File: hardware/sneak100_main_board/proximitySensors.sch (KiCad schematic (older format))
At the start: 29 parts, among them Q1 Q_Photo_NPN_CE, U1 CD4051B, U2 CD4051B

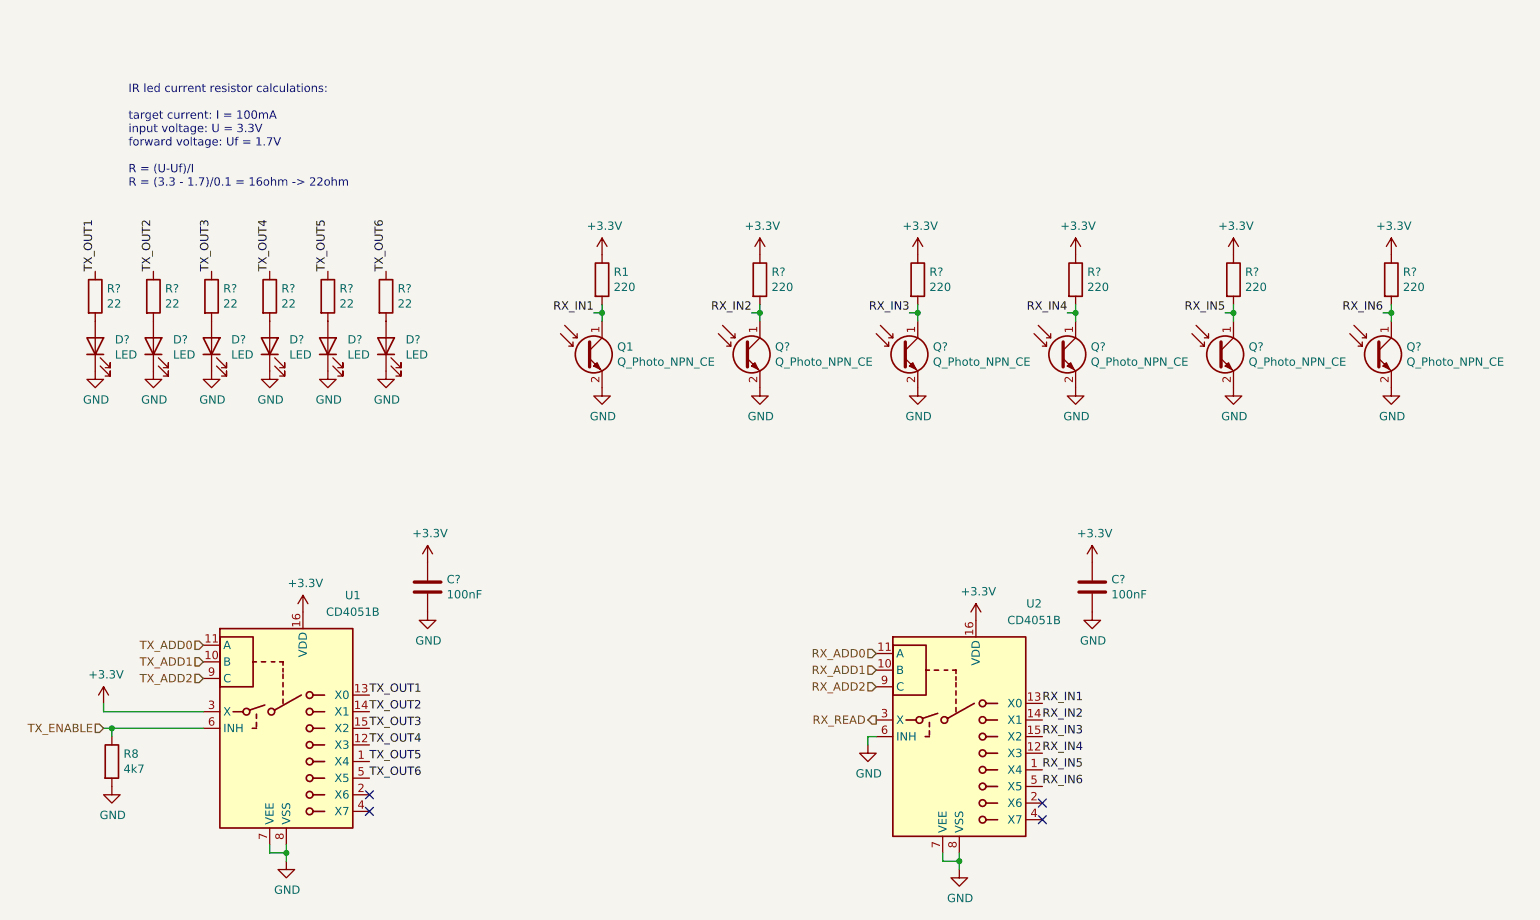
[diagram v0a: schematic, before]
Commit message: Proximity sensor first test
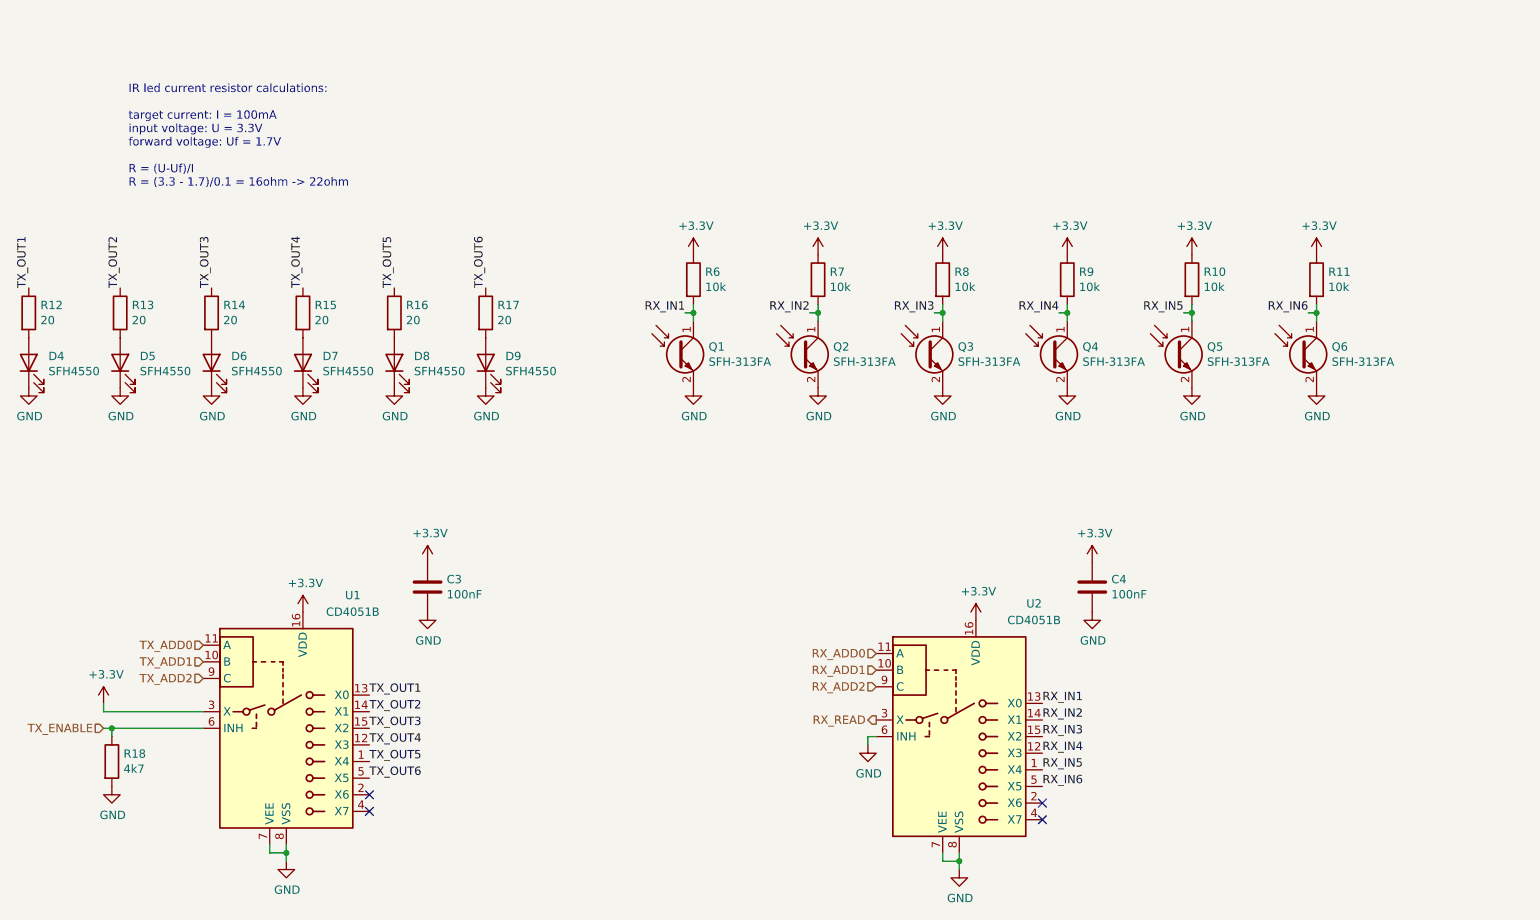
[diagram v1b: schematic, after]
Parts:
- D4, D5, D6, D7, D8, D9: renamed from D?; value LED -> SFH4550
- Q1: value Q_Photo_NPN_CE -> SFH-313FA
- Q2, Q3, Q4, Q5, Q6: renamed from Q?; value Q_Photo_NPN_CE -> SFH-313FA
- R10, R11, R7, R8, R9: renamed from R?; value 220 -> 10k
- R12, R13, R14, R15, R16, R17: renamed from R?; value 22 -> 20
- R6: renamed from R1; value 220 -> 10k
- gave numbers to parts that had none: 2
- renumbered R8 to R18
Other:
- moved on the sheet: D4, D5, D6, D7, D8, D9, Q1, Q2, Q3, Q4, Q5, Q6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

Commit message: motors circuit scheme
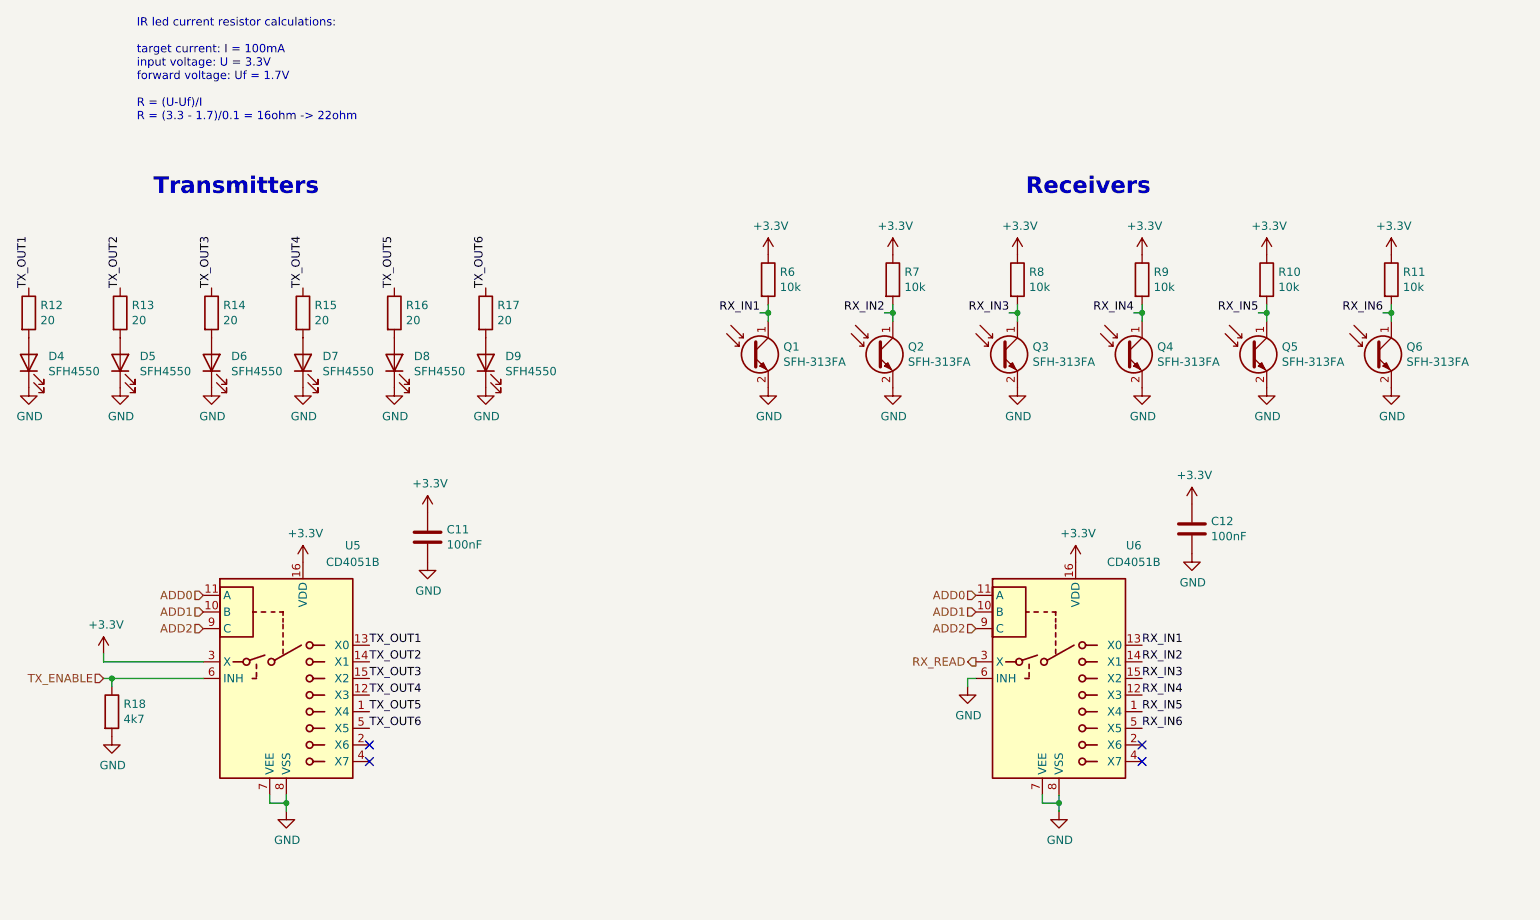
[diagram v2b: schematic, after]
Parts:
- C11: renamed from C3; footprint (none) -> Capacitor_SMD:C_0805_2012Metric
- C12: renamed from C4; footprint (none) -> Capacitor_SMD:C_0805_2012Metric
- D4, D5, D6, D7, D8, D9, Q1, Q2, Q3, Q4, Q5, Q6: footprint (none) -> Connector_PinHeader_2.54mm:PinHeader_1x02_P2.54mm_Vertical
- R10, R11, R12, R13, R14, R15, R16, R17, R18, R6, R7, R8, R9: footprint (none) -> Resistor_SMD:R_0805_2012Metric
- U5: renamed from U1; footprint (none) -> Package_SO:SOIC-16_3.9x9.9mm_P1.27mm
- U6: renamed from U2; footprint (none) -> Package_SO:SOIC-16_3.9x9.9mm_P1.27mm
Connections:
- net TX_ADD0 is gone; now on net ADD0: U5.11 (A)
- net TX_ADD1 is gone; now on net ADD1: U5.10 (B)
- net TX_ADD2 is gone; now on net ADD2: U5.9 (C)
- net RX_ADD0 renamed ADD0
- net RX_ADD1 renamed ADD1
- net RX_ADD2 renamed ADD2
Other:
- note added: "Receivers"
- note added: "Transmitters"
- moved on the sheet: C11, C12, Q1, Q2, Q3, Q4, Q5, Q6, R10, R11, R18, R6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
